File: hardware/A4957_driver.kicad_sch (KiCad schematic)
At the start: 21 parts, among them Q1 PSMN1R0-30YLC,115, Q2 PSMN1R0-30YLC,115, Q3 PSMN1R0-30YLC,115, Q4 PSMN1R0-30YLC,115

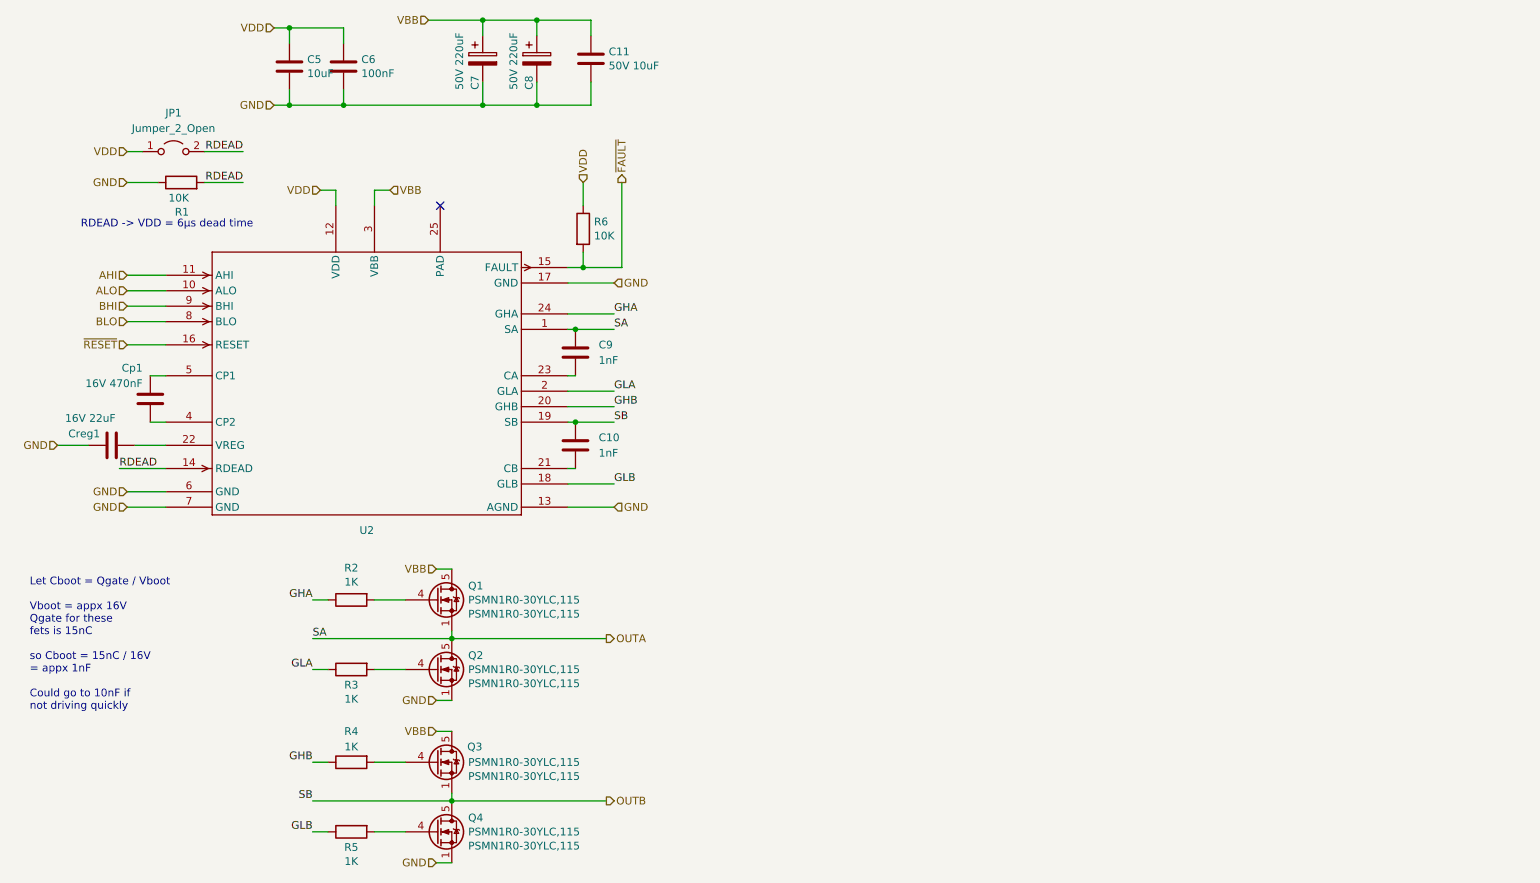
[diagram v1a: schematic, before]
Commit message: removed old
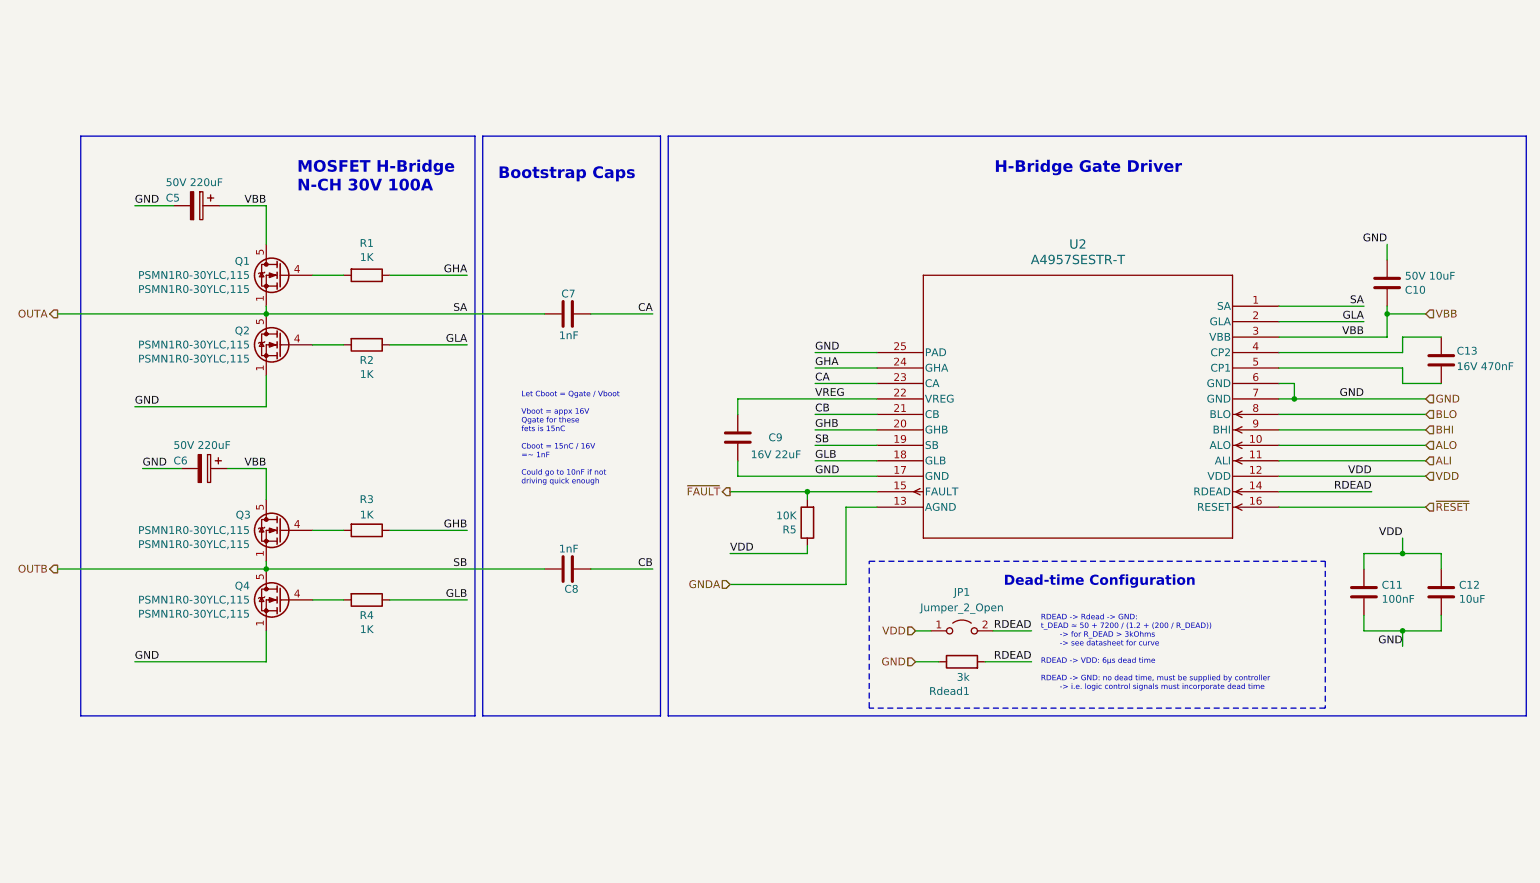
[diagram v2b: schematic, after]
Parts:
- removed Cp1: 16V 470nF, Capacitor_SMD:C_0805_2012Metric, symbol Device:C
- removed Creg1: 16V 22uF, Capacitor_SMD:C_0805_2012Metric, symbol Device:C
- removed U2: ~, Package_DFN_QFN:HVQFN-24-1EP_4x4mm_P0.5mm_EP2.6x2.6mm_ThermalVias, symbol DMATS_capstone:A4957
- added C13: 16V 470nF, Capacitor_SMD:C_0805_2012Metric_Pad1.18x1.45mm_HandSolder, symbol Device:C
- added C9: 16V 22uF, Capacitor_SMD:C_0805_2012Metric_Pad1.18x1.45mm_HandSolder, symbol Device:C
- added U2: A4957SESTR-T, kml-custom:QFN-24_ALM, symbol kml-custom:A4957SESTR-T
- C10: renamed from C11; footprint Capacitor_SMD:C_0805_2012Metric -> Capacitor_SMD:C_0805_2012Metric_Pad1.18x1.45mm_HandSolder
- C11: renamed from C6; footprint Capacitor_SMD:C_0805_2012Metric -> Capacitor_SMD:C_0805_2012Metric_Pad1.18x1.45mm_HandSolder
- C12: renamed from C5; footprint Capacitor_SMD:C_0805_2012Metric -> Capacitor_SMD:C_0805_2012Metric_Pad1.18x1.45mm_HandSolder
- C7: renamed from C9; footprint Capacitor_SMD:C_0805_2012Metric -> Capacitor_SMD:C_0805_2012Metric_Pad1.18x1.45mm_HandSolder
- C8: renamed from C10; footprint Capacitor_SMD:C_0805_2012Metric -> Capacitor_SMD:C_0805_2012Metric_Pad1.18x1.45mm_HandSolder
- R1: renamed from R2; footprint Capacitor_SMD:C_0805_2012Metric -> Resistor_SMD:R_0805_2012Metric_Pad1.20x1.40mm_HandSolder
- R2: renamed from R3; footprint Capacitor_SMD:C_0805_2012Metric -> Resistor_SMD:R_0805_2012Metric_Pad1.20x1.40mm_HandSolder
- R3: renamed from R4; footprint Capacitor_SMD:C_0805_2012Metric -> Resistor_SMD:R_0805_2012Metric_Pad1.20x1.40mm_HandSolder
- R4: renamed from R5; footprint Capacitor_SMD:C_0805_2012Metric -> Resistor_SMD:R_0805_2012Metric_Pad1.20x1.40mm_HandSolder
- R5: renamed from R6; footprint Capacitor_SMD:C_0805_2012Metric -> Resistor_SMD:R_0805_2012Metric_Pad1.20x1.40mm_HandSolder
- Rdead1: renamed from R1; value 10K -> 3k; footprint Capacitor_SMD:C_0805_2012Metric -> Resistor_SMD:R_0805_2012Metric_Pad1.20x1.40mm_HandSolder
- renumbered C7 to C5, C8 to C6
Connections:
- net ALO: now also U2.10 (ALO)
- net BHI: now also U2.9 (BHI)
- net BLO: now also U2.8 (BLO)
- net GHA: now also U2.24 (GHA)
- net GHB: now also U2.20 (GHB)
- net GLA: now also U2.2 (GLA)
- net GLB: now also U2.18 (GLB)
- net GND: now also C9.2, U2.17 (GND), U2.25 (PAD), U2.6 (GND), U2.7 (GND)
- net OUTA: now also U2.1 (SA)
- net OUTB: now also U2.19 (SB)
- net RDEAD: now also U2.14 (RDEAD)
- net VBB: now also U2.3 (VBB)
- net VDD: now also U2.12 (VDD)
- net ~{FAULT}: now also U2.15 (FAULT)
- net ~{RESET}: now also U2.16 (RESET)
- net CB: now reaches C8.2
- net CB: now also U2.21 (CB)
- net CA: now reaches C7.2
- net CA: now also U2.23 (CA)
- new net: C13.2, U2.4 (CP2)
- new net: C13.1, U2.5 (CP1)
- new net ALI: U2.11 (ALI)
- new net GNDA: U2.13 (AGND)
- new net VREG: C9.1, U2.22 (VREG)
- no-connect marks 1 -> 0
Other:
- note added: "Bootstrap Caps"
- note added: "Dead-time Configuration"
- note added: "H-Bridge Gate Driver"
- note added: "Let Cboot = Qgate / Vboot Vboot = appx 16V Qgate for these fets is 15nC Cboot = 15nC / 16V =~ 1nF Could go to 10nF if not driving quick enough"
- note added: "MOSFET H-Bridge N-CH 30V 100A"
- note added: "RDEAD -> Rdead -> GND: t_DEAD ≈ 50 + 7200 / (1.2 + (200 / R_DEAD)) -> for R_DEAD > 3kOhms -> see datasheet for curve RDEAD -> VDD: 6µs dead time RDEAD -> GND: no dead time, must be supplied by controller -> i.e. logic control signals must incorporate dead time"
- note removed: "Let Cboot = Qgate / Vboot Vboot = appx 16V Qgate for these fets is 15nC so Cboot = 15nC / 16V = appx 1nF Could go to 10nF if not driving quickly"
- note removed: "RDEAD -> VDD = 6µs dead time"
- moved on the sheet: C10, C11, C12, C5, C6, C7, C8, JP1, Q1, Q2, Q3, Q4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
